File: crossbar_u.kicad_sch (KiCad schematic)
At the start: 48 parts, among them U60 AD5160, U61 AD5160, U62 AD5160, U63 AD5160, U64 AD5160, U65 AD5160, U66 AD5160, U67 AD5160, U68 AD5160, U69 AD5160, U70 AD5160, U71 AD5160, U72 AD5160, U73 AD5160, U74 AD5160, U75 AD5160, U76 AD5160, U77 AD5160, U78 AD5160, U79 AD5160, U80 AD5160, U81 AD5160, U82 AD5160, U83 AD5160

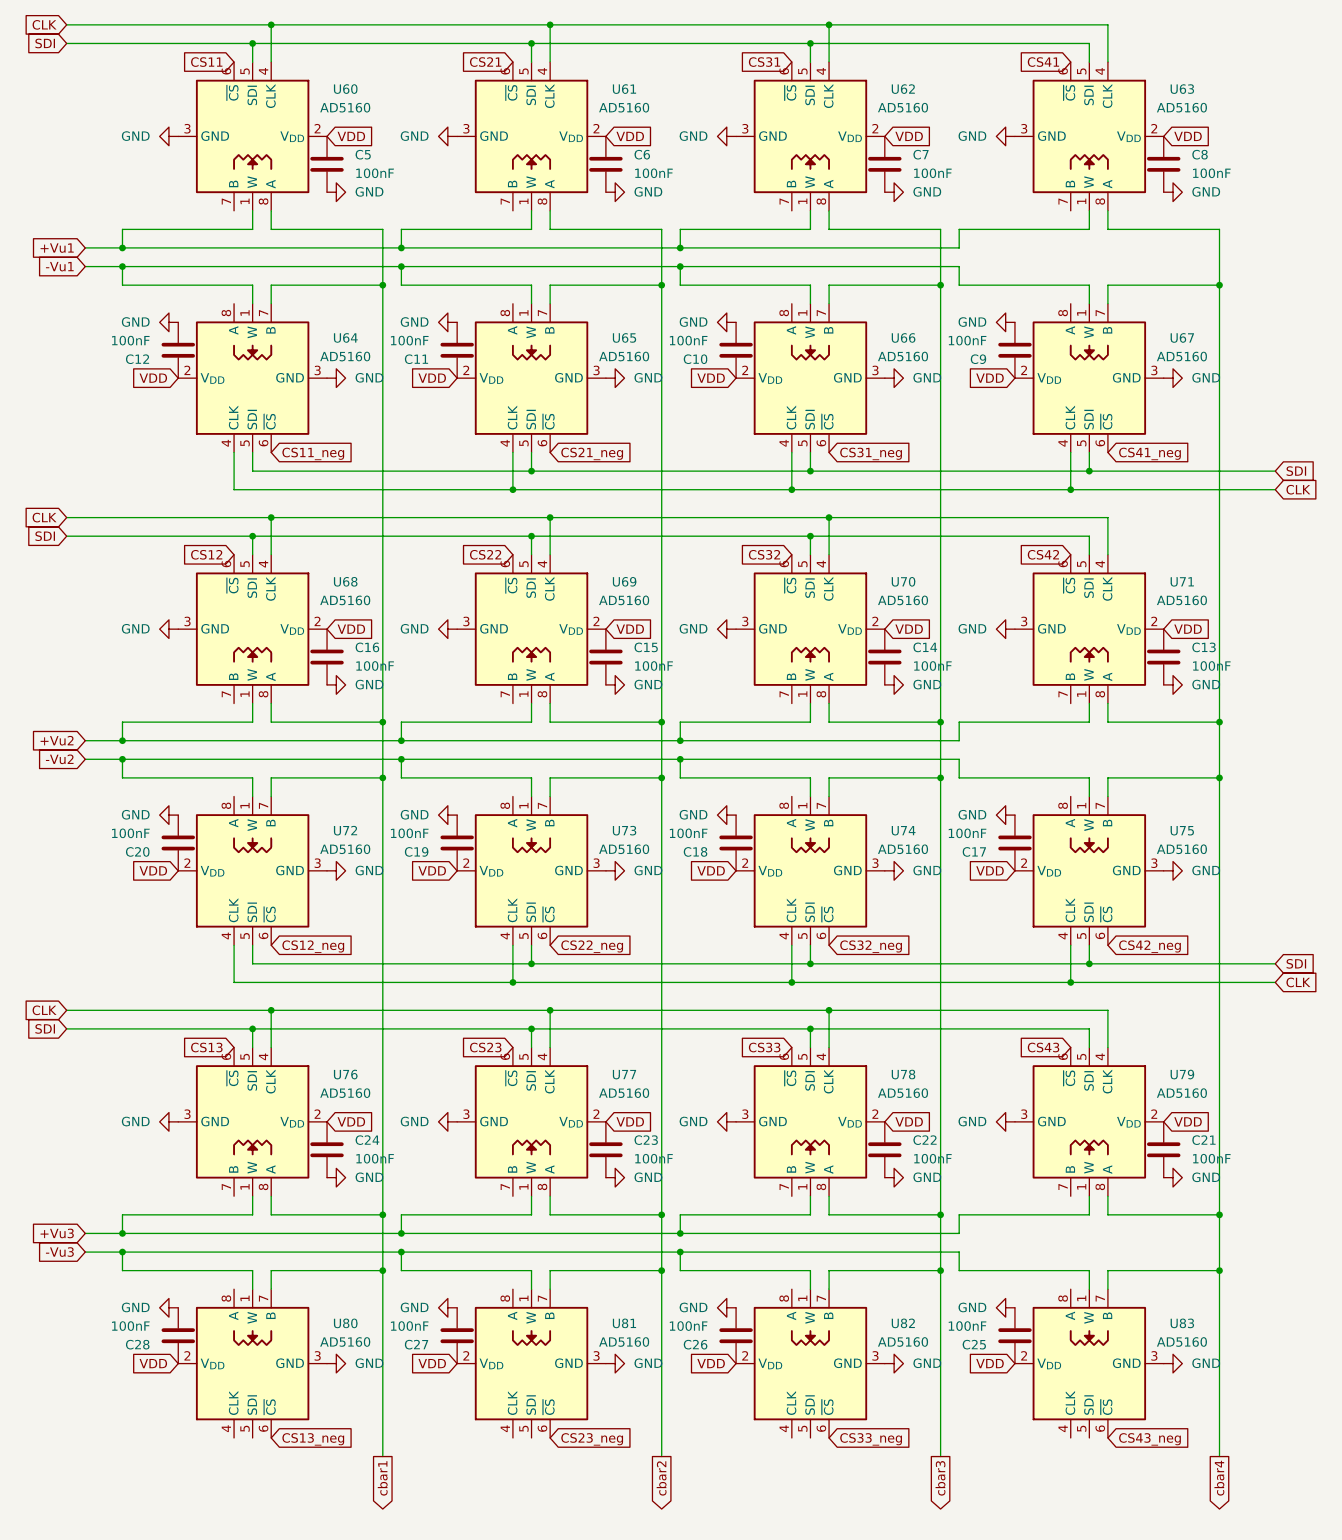
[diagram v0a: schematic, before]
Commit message: Updated: power
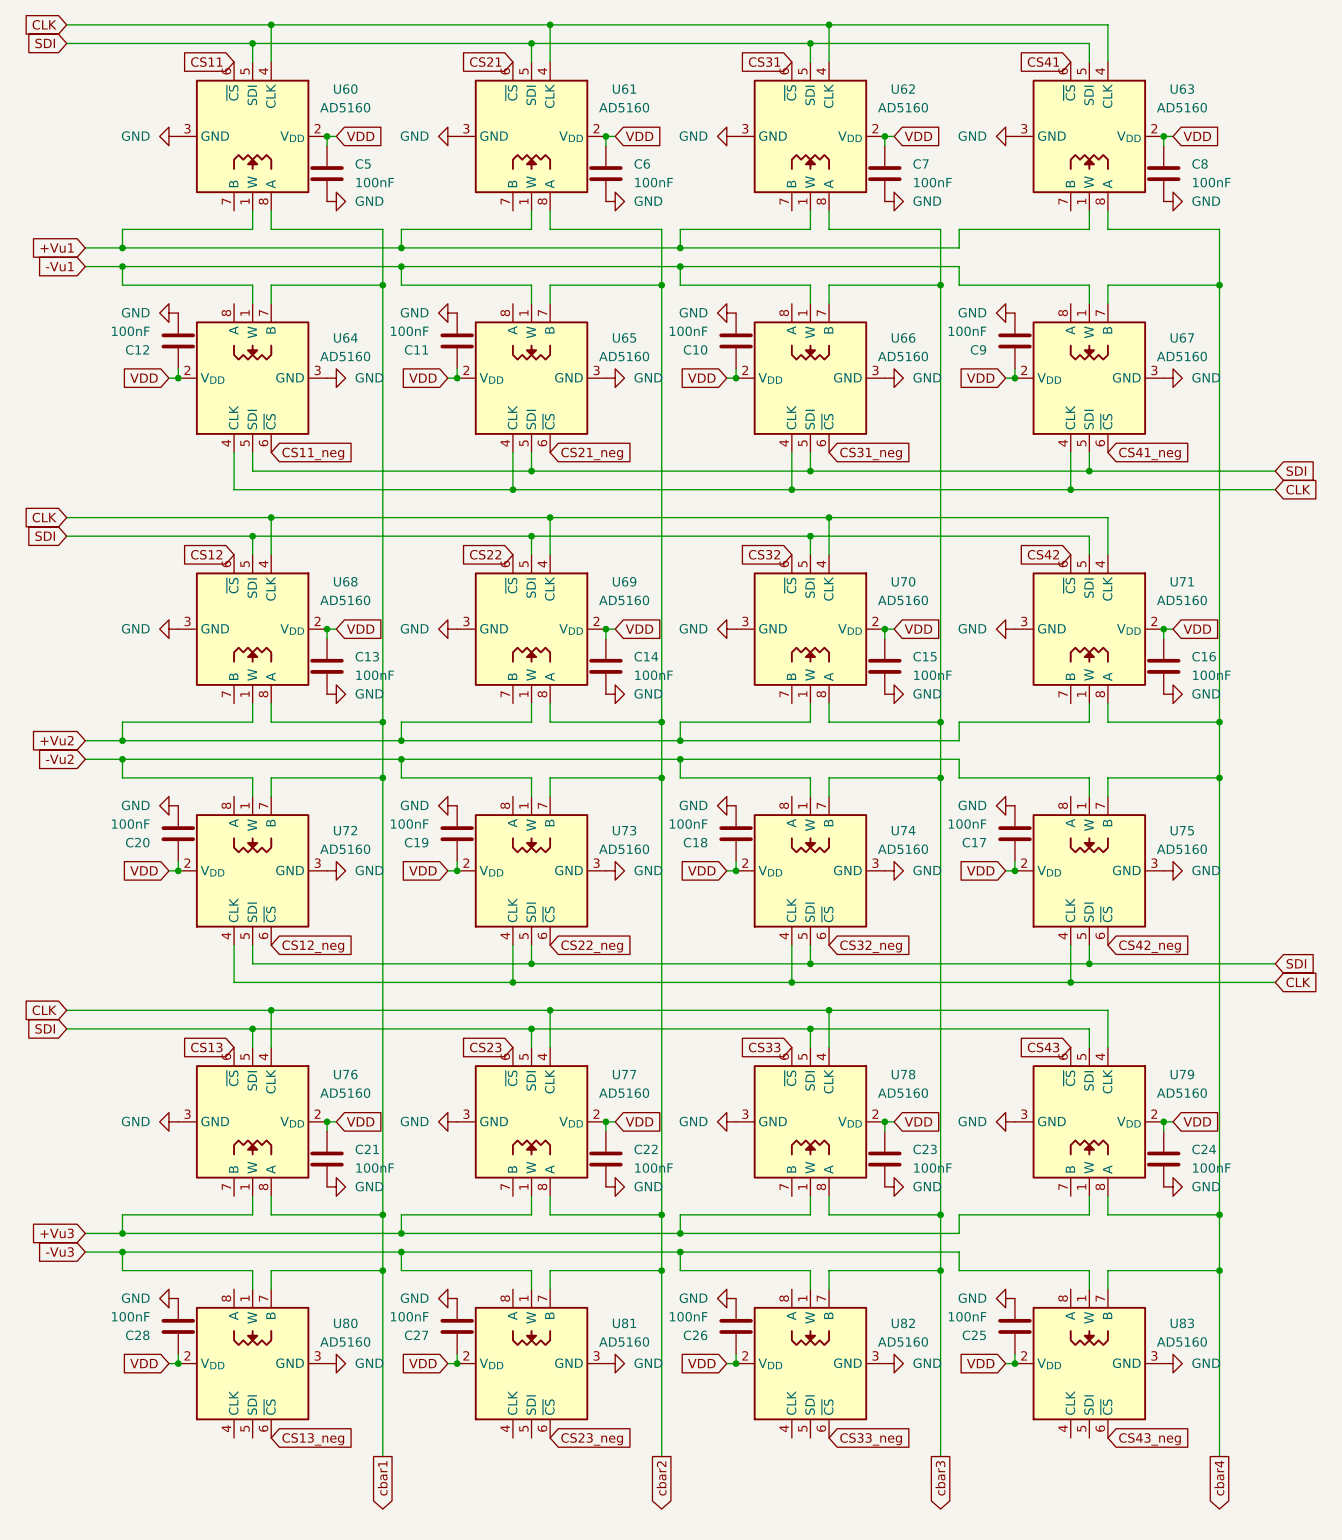
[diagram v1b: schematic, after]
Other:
- moved on the sheet: C5

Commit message: Updated: op amps
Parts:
- C10, C11, C12, C13, C14, C15, C16, C17, C18, C19, C20, C21, C22, C23, C24, C25, C26, C27, C28, C5, C6, C7, C8, C9: footprint (none) -> Capacitor_SMD:C_1206_3216Metric_Pad1.33x1.80mm_HandSolder
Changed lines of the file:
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@@
 			)
 		)
-		(property "Footprint" ""
+		(property "Footprint" "Capacitor_SMD:C_1206_3216Metric_Pad1.33x1.80mm_HandSolder"
 			(at 174.9552 128.27 0)
 			(effects
@@
 			)
 		)
-		(property "Footprint" ""
+		(property "Footprint" "Capacitor_SMD:C_1206_3216Metric_Pad1.33x1.80mm_HandSolder"
 			(at 76.5048 76.2 0)
 			(effects
@@
 			)
 		)
-		(property "Footprint" ""
+		(property "Footprint" "Capacitor_SMD:C_1206_3216Metric_Pad1.33x1.80mm_HandSolder"
 			(at 98.7552 60.96 0)
 			(effects
@@
 			)
 		)
-		(property "Footprint" ""
+		(property "Footprint" "Capacitor_SMD:C_1206_3216Metric_Pad1.33x1.80mm_HandSolder"
 			(at 114.6048 143.51 0)
 			(effects
@@
 			)
 		)
-		(property "Footprint" ""
+		(property "Footprint" "Capacitor_SMD:C_1206_3216Metric_Pad1.33x1.80mm_HandSolder"
 			(at 38.4048 143.51 0)
 			(effects
@@
 			)
 		)
-		(property "Footprint" ""
+		(property "Footprint" "Capacitor_SMD:C_1206_3216Metric_Pad1.33x1.80mm_HandSolder"
 			(at 60.6552 195.58 0)
 			(effects
@@
 			)
 		)
-		(property "Footprint" ""
+		(property "Footprint" "Capacitor_SMD:C_1206_3216Metric_Pad1.33x1.80mm_HandSolder"
 			(at 136.8552 60.96 0)
 			(effects
@@
 			)
 		)
-		(property "Footprint" ""
+		(property "Footprint" "Capacitor_SMD:C_1206_3216Metric_Pad1.33x1.80mm_HandSolder"
 			(at 136.8552 195.58 0)
 			(effects
@@
 			)
 		)
-		(property "Footprint" ""
+		(property "Footprint" "Capacitor_SMD:C_1206_3216Metric_Pad1.33x1.80mm_HandSolder"
 			(at 114.6048 76.2 0)
 			(effects
@@
 			)
 		)
-		(property "Footprint" ""
+		(property "Footprint" "Capacitor_SMD:C_1206_3216Metric_Pad1.33x1.80mm_HandSolder"
 			(at 114.6048 210.82 0)
 			(effects
@@
 			)
 		)
-		(property "Footprint" ""
+		(property "Footprint" "Capacitor_SMD:C_1206_3216Metric_Pad1.33x1.80mm_HandSolder"
 			(at 38.4048 76.2 0)
 			(effects
@@
 			)
 		)
-		(property "Footprint" ""
+		(property "Footprint" "Capacitor_SMD:C_1206_3216Metric_Pad1.33x1.80mm_HandSolder"
 			(at 136.8552 128.27 0)
 			(effects
@@
 			)
 		)
-		(property "Footprint" ""
+		(property "Footprint" "Capacitor_SMD:C_1206_3216Metric_Pad1.33x1.80mm_HandSolder"
 			(at 38.4048 210.82 0)
 			(effects
@@
 			)
 		)
-		(property "Footprint" ""
+		(property "Footprint" "Capacitor_SMD:C_1206_3216Metric_Pad1.33x1.80mm_HandSolder"
 			(at 98.7552 128.27 0)
 			(effects
@@
 			)
 		)
-		(property "Footprint" ""
+		(property "Footprint" "Capacitor_SMD:C_1206_3216Metric_Pad1.33x1.80mm_HandSolder"
 			(at 174.9552 60.96 0)
 			(effects
@@
 			)
 		)
-		(property "Footprint" ""
+		(property "Footprint" "Capacitor_SMD:C_1206_3216Metric_Pad1.33x1.80mm_HandSolder"
 			(at 76.5048 210.82 0)
 			(effects
@@
 			)
 		)
-		(property "Footprint" ""
+		(property "Footprint" "Capacitor_SMD:C_1206_3216Metric_Pad1.33x1.80mm_HandSolder"
 			(at 152.7048 76.2 0)
 			(effects
@@
 			)
 		)
-		(property "Footprint" ""
+		(property "Footprint" "Capacitor_SMD:C_1206_3216Metric_Pad1.33x1.80mm_HandSolder"
 			(at 152.7048 143.51 0)
 			(effects
@@
 			)
 		)
-		(property "Footprint" ""
+		(property "Footprint" "Capacitor_SMD:C_1206_3216Metric_Pad1.33x1.80mm_HandSolder"
 			(at 60.6552 60.96 0)
 			(effects
@@
 			)
 		)
-		(property "Footprint" ""
+		(property "Footprint" "Capacitor_SMD:C_1206_3216Metric_Pad1.33x1.80mm_HandSolder"
 			(at 152.7048 210.82 0)
 			(effects
@@
 			)
 		)
-		(property "Footprint" ""
+		(property "Footprint" "Capacitor_SMD:C_1206_3216Metric_Pad1.33x1.80mm_HandSolder"
 			(at 60.6552 128.27 0)
 			(effects
@@
 			)
 		)
-		(property "Footprint" ""
+		(property "Footprint" "Capacitor_SMD:C_1206_3216Metric_Pad1.33x1.80mm_HandSolder"
 			(at 98.7552 195.58 0)
 			(effects
@@
 			)
 		)
-		(property "Footprint" ""
+		(property "Footprint" "Capacitor_SMD:C_1206_3216Metric_Pad1.33x1.80mm_HandSolder"
 			(at 76.5048 143.51 0)
 			(effects
@@
 			)
 		)
-		(property "Footprint" ""
+		(property "Footprint" "Capacitor_SMD:C_1206_3216Metric_Pad1.33x1.80mm_HandSolder"
 			(at 174.9552 195.58 0)
 			(effects
